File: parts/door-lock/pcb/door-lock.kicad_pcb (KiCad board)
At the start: 2 copper layers, 63.2 x 40 mm, 13 parts, among them J2 RJ45_Shielded, U1 L293D

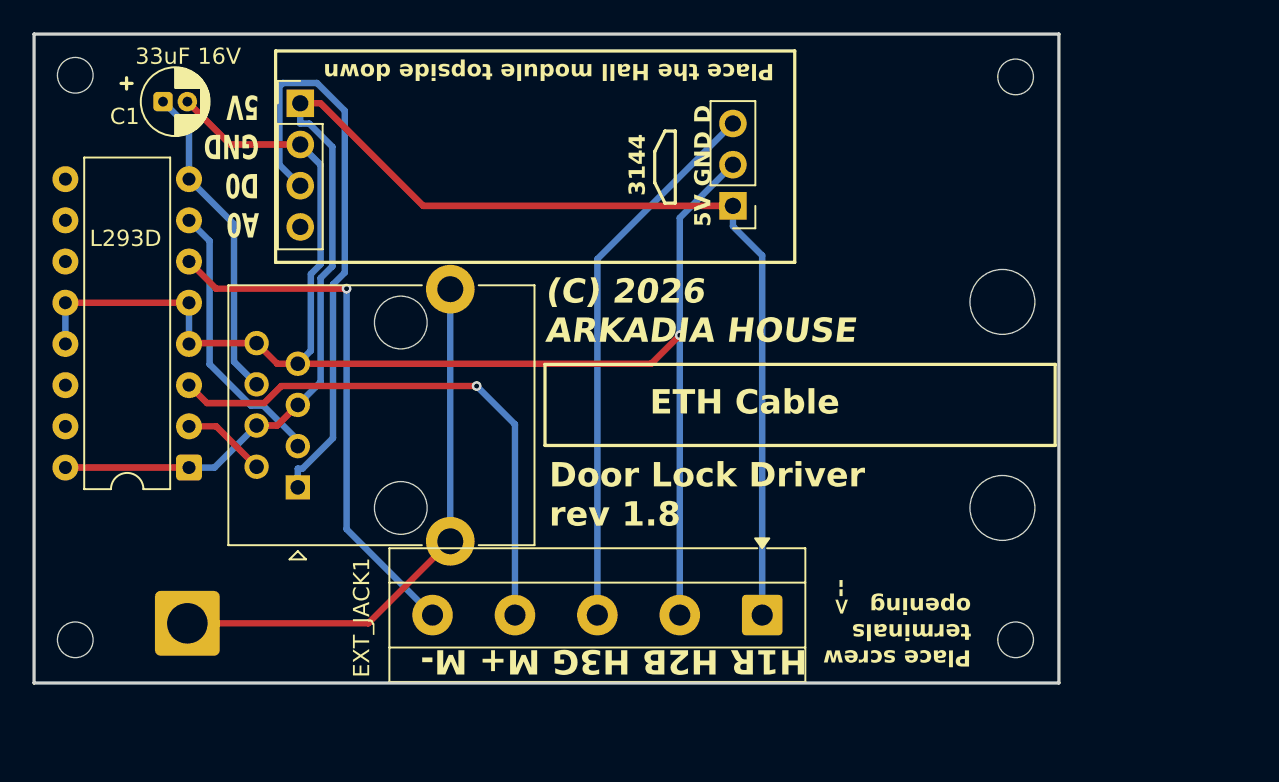
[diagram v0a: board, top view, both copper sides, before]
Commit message: door lock refinements.
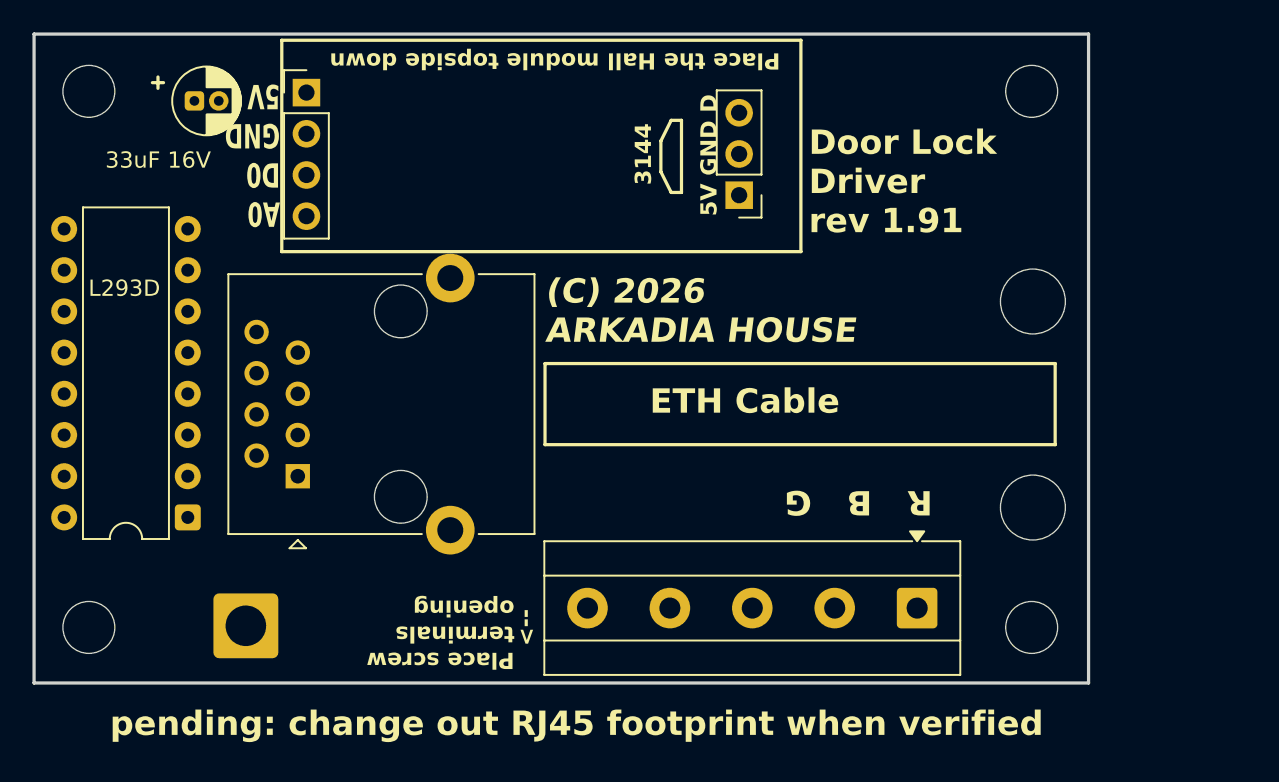
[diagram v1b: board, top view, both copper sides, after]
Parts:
- mh1, mh2, mh3, mh4: value MountingHole_2.2mm_M2 -> MountingHole_3.2mm_M3; footprint MountingHole:MountingHole_2.2mm_M2 -> MountingHole:MountingHole_3.2mm_M3
- moved EXT_JACK1 9.56 mm to (117.9, 58.2)
- moved SHIELD1 3.61 mm to (76.6, 59.3)
- moved U1 3.07 mm to (73.0, 52.7)
- moved C1 1.94 mm to (73.4, 27.0)
- moved ziptie_hole1 1.88 mm to (125.1, 39.3)
- moved ziptie_hole2 1.88 mm to (125.1, 52.0)
- moved mh3 1.33 mm to (125.0, 26.4)
- moved mh1 1.30 mm to (66.9, 26.4)
- moved mh4 1.25 mm to (125.0, 59.4)
- moved mh2 1.13 mm to (66.9, 59.4)
- moved HALL_MODULE_PT1 0.76 mm to (80.3, 26.5)
- moved HALL_MODULE_PT2 0.76 mm to (107.0, 32.8)
- moved J2 0.69 mm to (79.8, 50.1)
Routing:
- net /GND: track 96.0 -> 0.00 mm, vias 1 -> 0
- net /5V: track 91.8 -> 0.00 mm
- net /SENSE: track 36.1 -> 0.00 mm
- net unconnected-(J2-PadSH): track 33.8 -> 0.00 mm
- net /OUT: track 33.8 -> 0.00 mm
- net Net-(EXT_JACK1-MOTOR+): track 33.7 -> 0.00 mm, vias 1 -> 0
- net Net-(EXT_JACK1-MOTOR-): track 32.7 -> 0.00 mm, vias 1 -> 0
- net /12V: track 19.8 -> 0.00 mm
- net /UNLOCK: track 17.1 -> 0.00 mm
- net /LOCK: track 5.20 -> 0.00 mm
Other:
- board size 63.2 x 40 mm -> 65 x 40 mm
- board text added: "Door Lock Driver rev 1.91"
- board text added: "R B G"
- board text added: "pending: change out RJ45 footprint when verified"
- board text removed: "Door Lock Driver rev 1.8"
- board text removed: "H1R H2B H3G M+ M-"
